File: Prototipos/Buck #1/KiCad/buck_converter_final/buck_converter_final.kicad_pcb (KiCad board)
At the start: 2 copper layers, 100 x 100 mm, 25 parts, among them J1 Conn_01x03_Pin, J3 Screw_Terminal_01x02, Q1 IRF9540NPBF, Q3 NPN

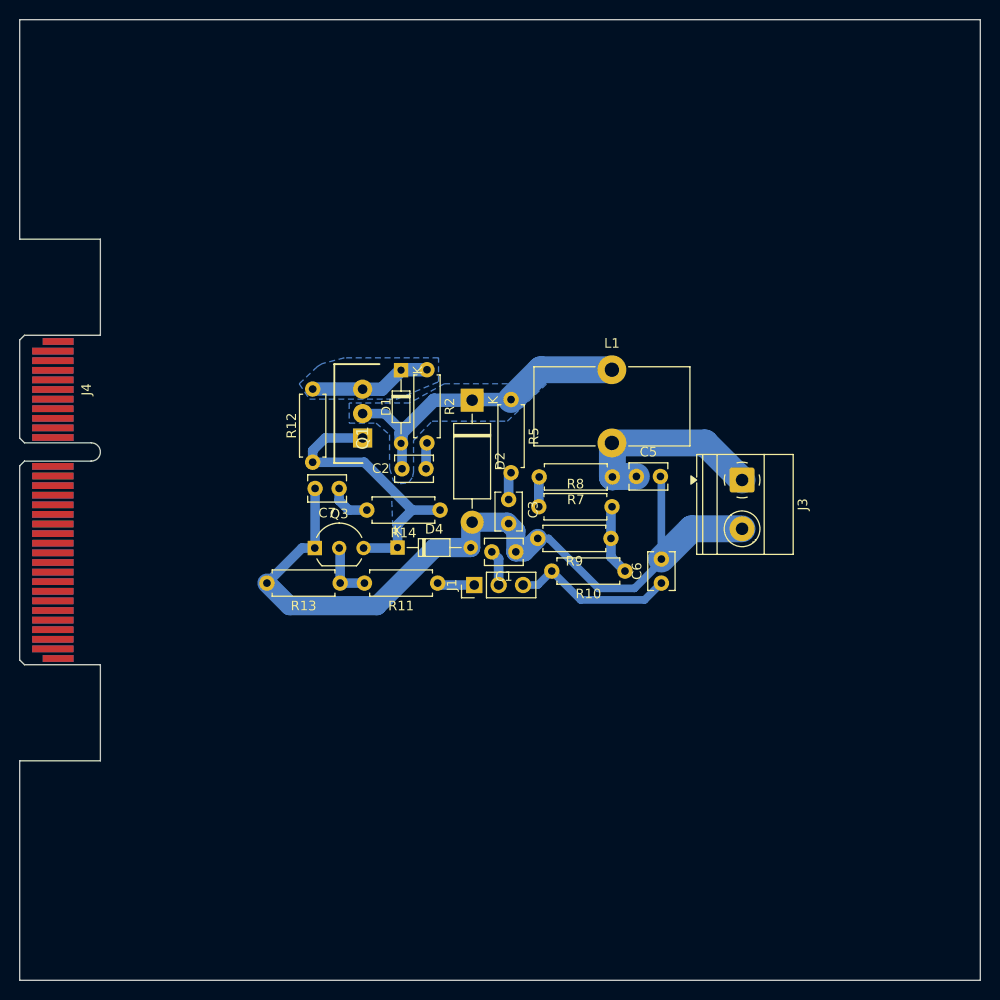
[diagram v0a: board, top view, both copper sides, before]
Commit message: Avances en PCB final buck, versión 1.1
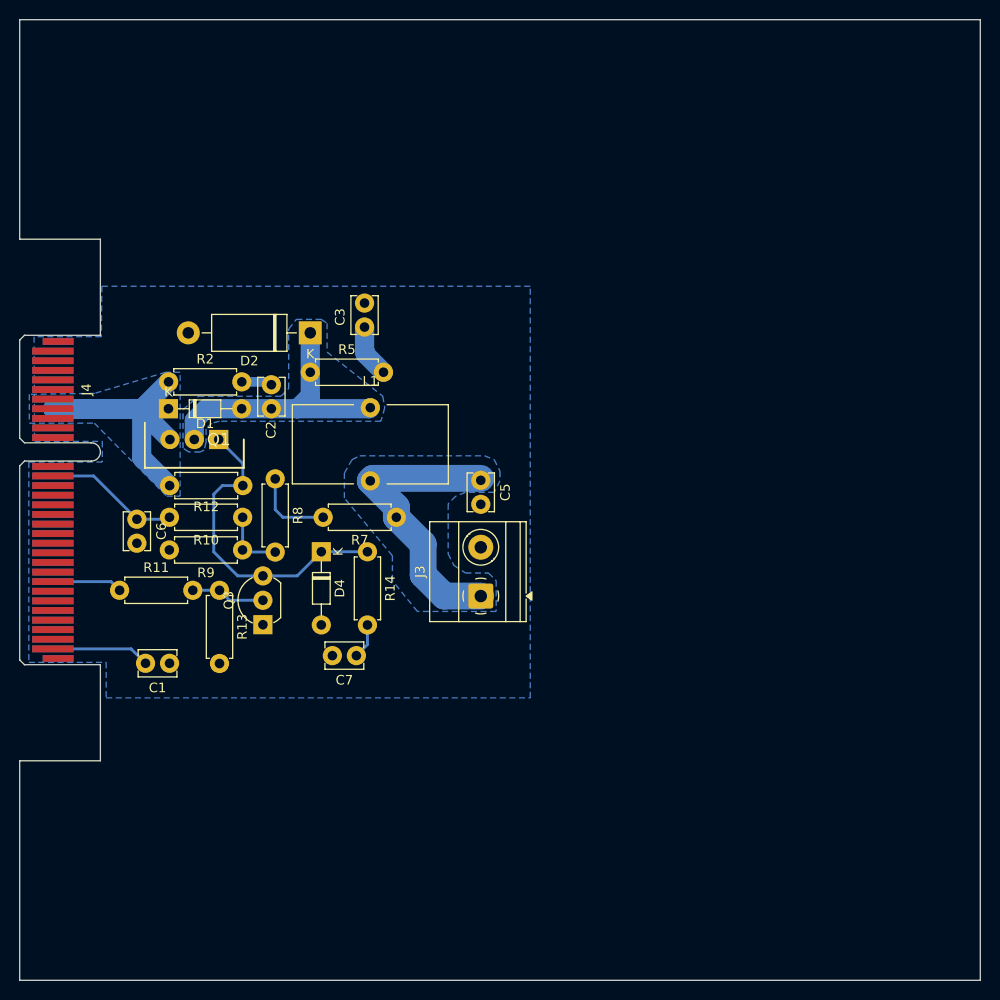
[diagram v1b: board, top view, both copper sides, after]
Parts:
- removed J1: Conn_01x03_Pin, Connector_PinHeader_2.54mm:PinHeader_1x03_P2.54mm_Vertical
- moved C6 55.0 mm to (117.0, 85.0), turned to -90 degrees
- moved R10 40.2 mm to (128.0, 84.8)
- moved R9 38.4 mm to (128.0, 88.2)
- moved C1 37.9 mm to (120.4, 100.0)
- moved R11 33.1 mm to (115.2, 92.4), turned to 0 degrees
- moved J3 29.8 mm to (152.8, 93.0), turned to 90 degrees
- moved R8 27.6 mm to (131.4, 80.8), turned to -90 degrees
- moved R2 26.9 mm to (120.3, 70.7), turned to 0 degrees
- moved L1 25.5 mm to (141.3, 73.4)
- moved D1 24.5 mm to (120.3, 73.5), turned to 0 degrees
- moved C3 23.4 mm to (140.7, 65.0), turned to 90 degrees
- moved R7 22.9 mm to (144.0, 84.8)
- moved R5 21.1 mm to (135.1, 69.7), turned to 0 degrees
- moved C2 18.3 mm to (131.0, 71.0), turned to -90 degrees
- moved D2 18.3 mm to (135.1, 65.6), turned to 180 degrees
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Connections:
- J4 pad 10: RETRO_MICRO -> unconnected-(J4-S4-Pad10)
- J4 pad 26: unconnected-(J4-S20-Pad26) -> PWM_CONTROL
- J4 pad 8: PWM_CONTROL -> RETRO_MICRO
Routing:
- net PGND: track 84.9 -> 0.00 mm
- net 12V: track 12.7 -> 48.0 mm
- net Net-(J3-Pin_1): track 21.2 -> 30.6 mm
- net AGND: track 3.74 -> 10.3 mm
- net Net-(R7-Pad2): track 3.12 -> 8.52 mm
- net Net-(D1-A): track 34.5 -> 29.6 mm
- net PWM_CONTROL: track 3.89 -> 7.32 mm
- net Gate: track 30.4 -> 33.3 mm
- net RETRO_MICRO: track 17.0 -> 14.1 mm
- net Net-(C3-Pad1): track 2.89 -> 5.52 mm
- net Net-(Q3-B): track 6.22 -> 7.73 mm
- net Net-(C7-Pad1): track 4.82 -> 3.67 mm
- added copper zone on B.Cu, net Net-(J3-Pin_1)
- added copper zone on B.Cu, net PGND
- removed copper zone on B.Cu, net Gate
